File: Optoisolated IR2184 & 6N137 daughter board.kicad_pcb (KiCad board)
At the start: 2 copper layers, 41.3 x 31.6 mm, 15 parts, among them J1 Screw_Terminal_01x08, U1 6N137, U2 IR2184, U3 LM78L05_TO92

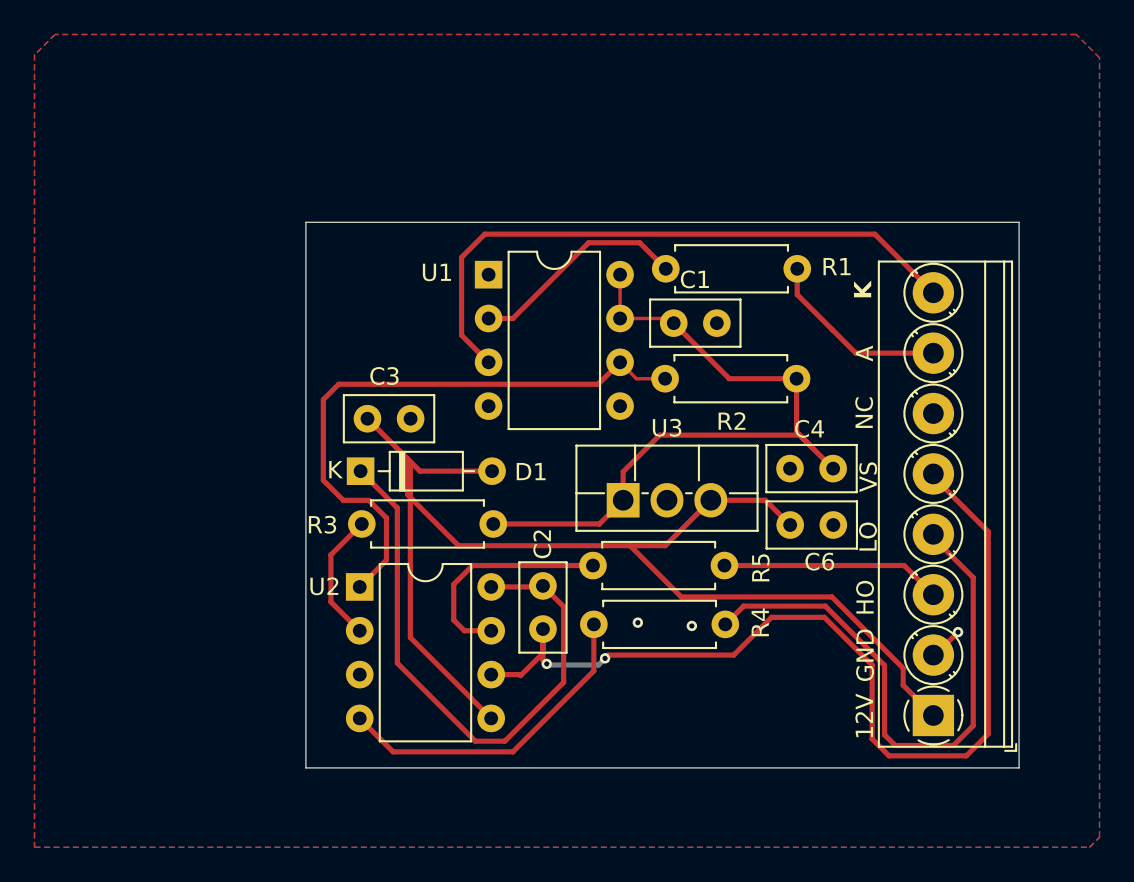
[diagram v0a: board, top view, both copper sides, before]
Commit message: Update project files
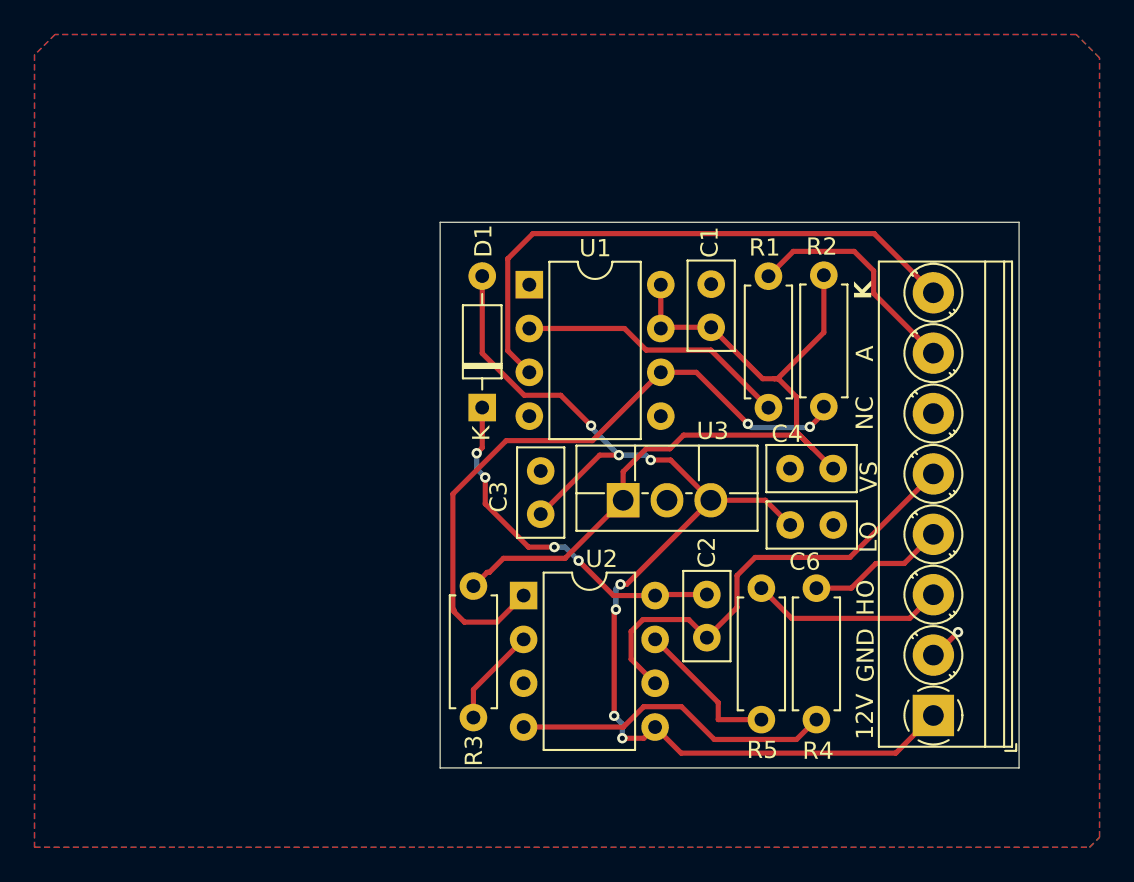
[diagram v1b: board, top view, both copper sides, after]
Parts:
- moved R4 14.0 mm to (206.1, 78.7), turned to 90 degrees
- moved R5 13.2 mm to (202.9, 78.7), turned to 90 degrees
- moved C3 11.5 mm to (190.1, 66.8), turned to 90 degrees
- moved C2 9.51 mm to (199.7, 71.4)
- moved U2 9.51 mm to (189.1, 71.5)
- moved R2 9.34 mm to (206.5, 60.5), turned to 90 degrees
- moved D1 7.96 mm to (186.7, 60.6), turned to 90 degrees
- moved R3 3.78 mm to (186.2, 70.9), turned to -90 degrees
- moved U1 2.43 mm to (189.4, 53.5)
- moved C1 2.18 mm to (200.0, 55.9), turned to 90 degrees
- moved R1 1.72 mm to (203.3, 53.0), turned to -90 degrees
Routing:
- net /VS: track 55.8 -> 26.8 mm, vias 2 -> 0
- net /LO: track 33.0 -> 8.07 mm
- net Net-(D1-K): track 34.0 -> 21.0 mm, vias 0 -> 4
- net /5V: track 42.2 -> 49.0 mm
- net /12V_VCC: track 74.7 -> 68.8 mm, vias 0 -> 7
- net /HO_R: track 13.0 -> 8.67 mm
- net /VO: track 35.0 -> 38.2 mm, vias 0 -> 2
- net Net-(U1-A): track 12.7 -> 15.8 mm
- net /OPT_A: track 10.8 -> 13.4 mm
- net /OPT_K(GND): track 36.2 -> 33.8 mm
- net Net-(U2-~{SD}): track 7.62 -> 5.74 mm
- net /HO: track 12.8 -> 11.3 mm
- net GND: vias 3 -> 1
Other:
- board size 41.3 x 31.6 mm -> 33.6 x 31.6 mm
